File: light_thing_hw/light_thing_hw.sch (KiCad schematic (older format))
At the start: 53 parts, among them J1 CONNECTORS, J2 Li-Ion Battery, J3 ADDR_LED_PANEL_1_CONNECTORS, J4 ADDR_LED_PANEL_2_CONNECTORS, Q1 MMBF170, SW1 ST_USER_BUTTON1, SW2 ST_RESET_BUTTON, U1 BC832-V1, U2 LSM6DS3, U3 MCP73833T-FCI_UN, U4 LMR62421XMF, U5 LP38511MRX-ADJ_NOPB, U5A1 STM32L452RETx

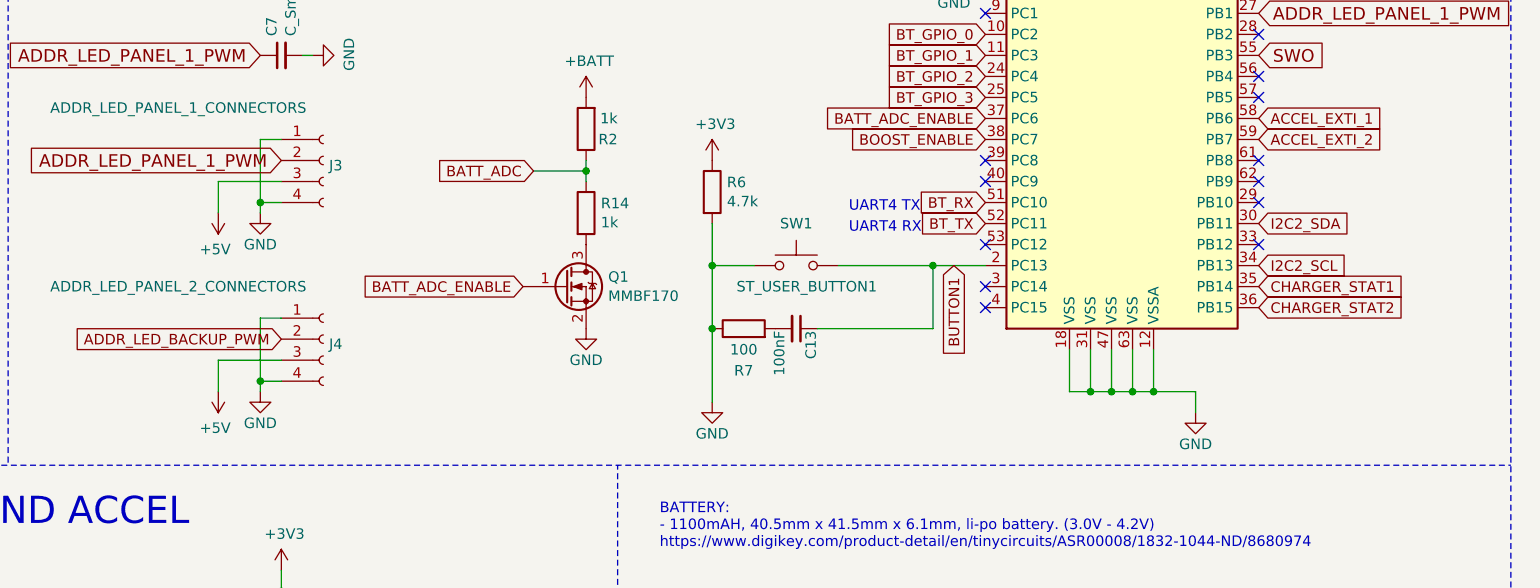
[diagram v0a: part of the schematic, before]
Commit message: restarting routing
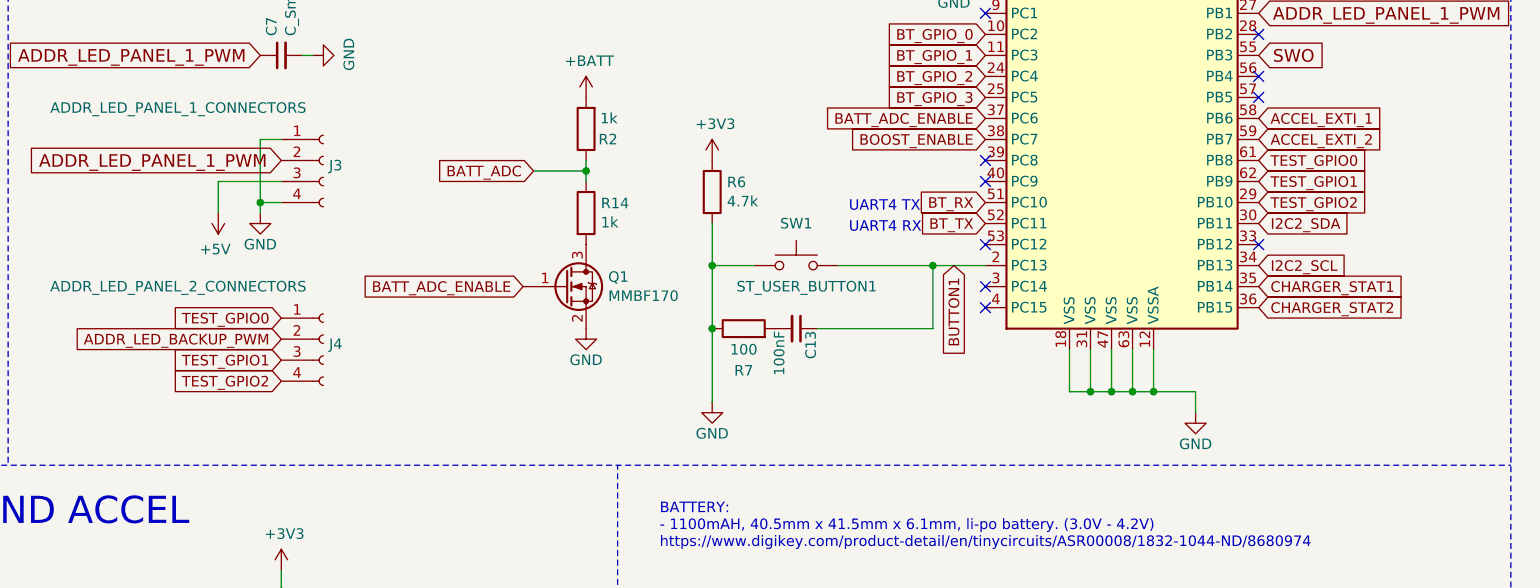
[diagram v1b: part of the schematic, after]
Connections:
- net +5V: no longer J4.3 (Pin_3)
- net GND: no longer J4.1 (Pin_1), J4.4 (Pin_4)
- net TEST_GPIO2: now reaches U5A1.29 (PB10)
- net TEST_GPIO2: now also J4.4 (Pin_4)
- net TEST_GPIO0: now reaches U5A1.61 (PB8)
- net TEST_GPIO0: now also J4.1 (Pin_1)
- net TEST_GPIO1: now reaches U5A1.62 (PB9)
- net TEST_GPIO1: now also J4.3 (Pin_3)
- no-connect marks 49 -> 46
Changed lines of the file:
@@
 	1    0    0    -1
 $EndComp
-$Comp
-L power:GND #PWR0112
-U 1 1 5F27037F
-P 5250 4850
-F 0 "#PWR0112" H 5250 4600 50  0001 C CNN
-F 1 "GND" H 5250 4700 50  0000 C CNN
-F 2 "" H 5250 4850 50  0001 C CNN
-F 3 "" H 5250 4850 50  0001 C CNN
-	1    5250 4850
-	1    0    0    -1
-$EndComp
-Wire Wire Line
-	5350 4500 5250 4500
-Wire Wire Line
-	5250 4500 5250 4800
-Wire Wire Line
-	5350 4800 5250 4800
-Connection ~ 5250 4800
-Wire Wire Line
-	5250 4800 5250 4850
-$Comp
-L power:+5V #PWR0113
-U 1 1 5F27038A
-P 5050 4850
-F 0 "#PWR0113" H 5050 4700 50  0001 C CNN
-F 1 "+5V" H 5065 5023 50  0000 C CNN
-F 2 "" H 5050 4850 50  0001 C CNN
-F 3 "" H 5050 4850 50  0001 C CNN
-	1    5050 4850
-	-1   0    0    1
-$EndComp
-Wire Wire Line
-	5350 4700 5050 4700
-Wire Wire Line
-	5050 4700 5050 4850
-Text GLabel 5350 4600 0    50   Input ~ 0
-ADDR_LED_BACKUP_PWM
 Text GLabel 10000 1750 2    50   Input ~ 0
 GREEN_LED
@@
 NoConn ~ 10000 3350
 NoConn ~ 10000 3450
-NoConn ~ 10000 3750
-NoConn ~ 10000 3850
-NoConn ~ 10000 4150
 NoConn ~ 8700 4450
 NoConn ~ 8700 4350
@@
 NoConn ~ 2600 1300
 NoConn ~ 1650 1500
-NoConn ~ 10000 3950
 Text GLabel 10000 4350 2    50   Input ~ 0
 CHARGER_STAT1
@@
 Wire Wire Line
 	2600 1700 3350 1700
+Text GLabel 10000 3750 2    50   Input ~ 0
+TEST_GPIO0
+Text GLabel 10000 3850 2    50   Input ~ 0
+TEST_GPIO1
+Text GLabel 10000 3950 2    50   Input ~ 0
+TEST_GPIO2
+Text GLabel 5350 4600 0    50   Input ~ 0
+ADDR_LED_BACKUP_PWM
+NoConn ~ 10000 4150
+Text GLabel 5350 4500 0    50   Input ~ 0
+TEST_GPIO0
+Text GLabel 5350 4700 0    50   Input ~ 0
+TEST_GPIO1
+Text GLabel 5350 4800 0    50   Input ~ 0
+TEST_GPIO2
 $EndSCHEMATC
